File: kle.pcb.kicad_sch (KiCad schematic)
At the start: 191 parts, among them J2 Conn_02x03_Odd_Even, K0 Esc, K1 F1, K10 F10, K11 F11, K12 F12, K13 PrtSc,NmLk, K14 Pause,ScrLk, K15 Delete,Insert, K16 ~~,`, K17 !,1, K18 @,2, K19 #,3, K2 F2, K20 $,4, K21 %,5, K22 ^,6, K23 &,7, K24 *,8, K25 (,9, K26 ),0, K27 _,-, K28 +,=, K29 Backspace, K3 F3, K30 Home, K31 Tab, K32 Q, K33 W, K34 E, K35 R, K36 T, K37 Y, K38 U, K39 I, K4 F4, K40 O, K41 P, K42 {,[, K43 },], K44 |,\, K45 Page Up, K46 Caps Lock, K47 A, K48 S, K49 D, K5 F5, K50 F, K51 G, K52 H, K53 J, K54 K, K55 L, K56 :,;, K57 ",', K58 Enter, K59 Page Down, K6 F6, K60 Shift, K61 Z, K62 X, K63 C, K64 V, K65 B, K66 N, K67 M, K68 <,,, K69 >,., K7 F7, K70 ?,/, K71 Shift, K72 ↑, K73 End, K74 Ctrl, K75 Win, K76 Alt, K77 Blank, K78 Alt, K79 Fn, K8 F8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

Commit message: initial commit
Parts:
- K77: value Blank -> Space
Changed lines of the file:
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@@
 			)
 		)
-		(property "Value" "Blank"
+		(property "Value" "Space"
 			(at 160.02 92.71 0)
 			(effects

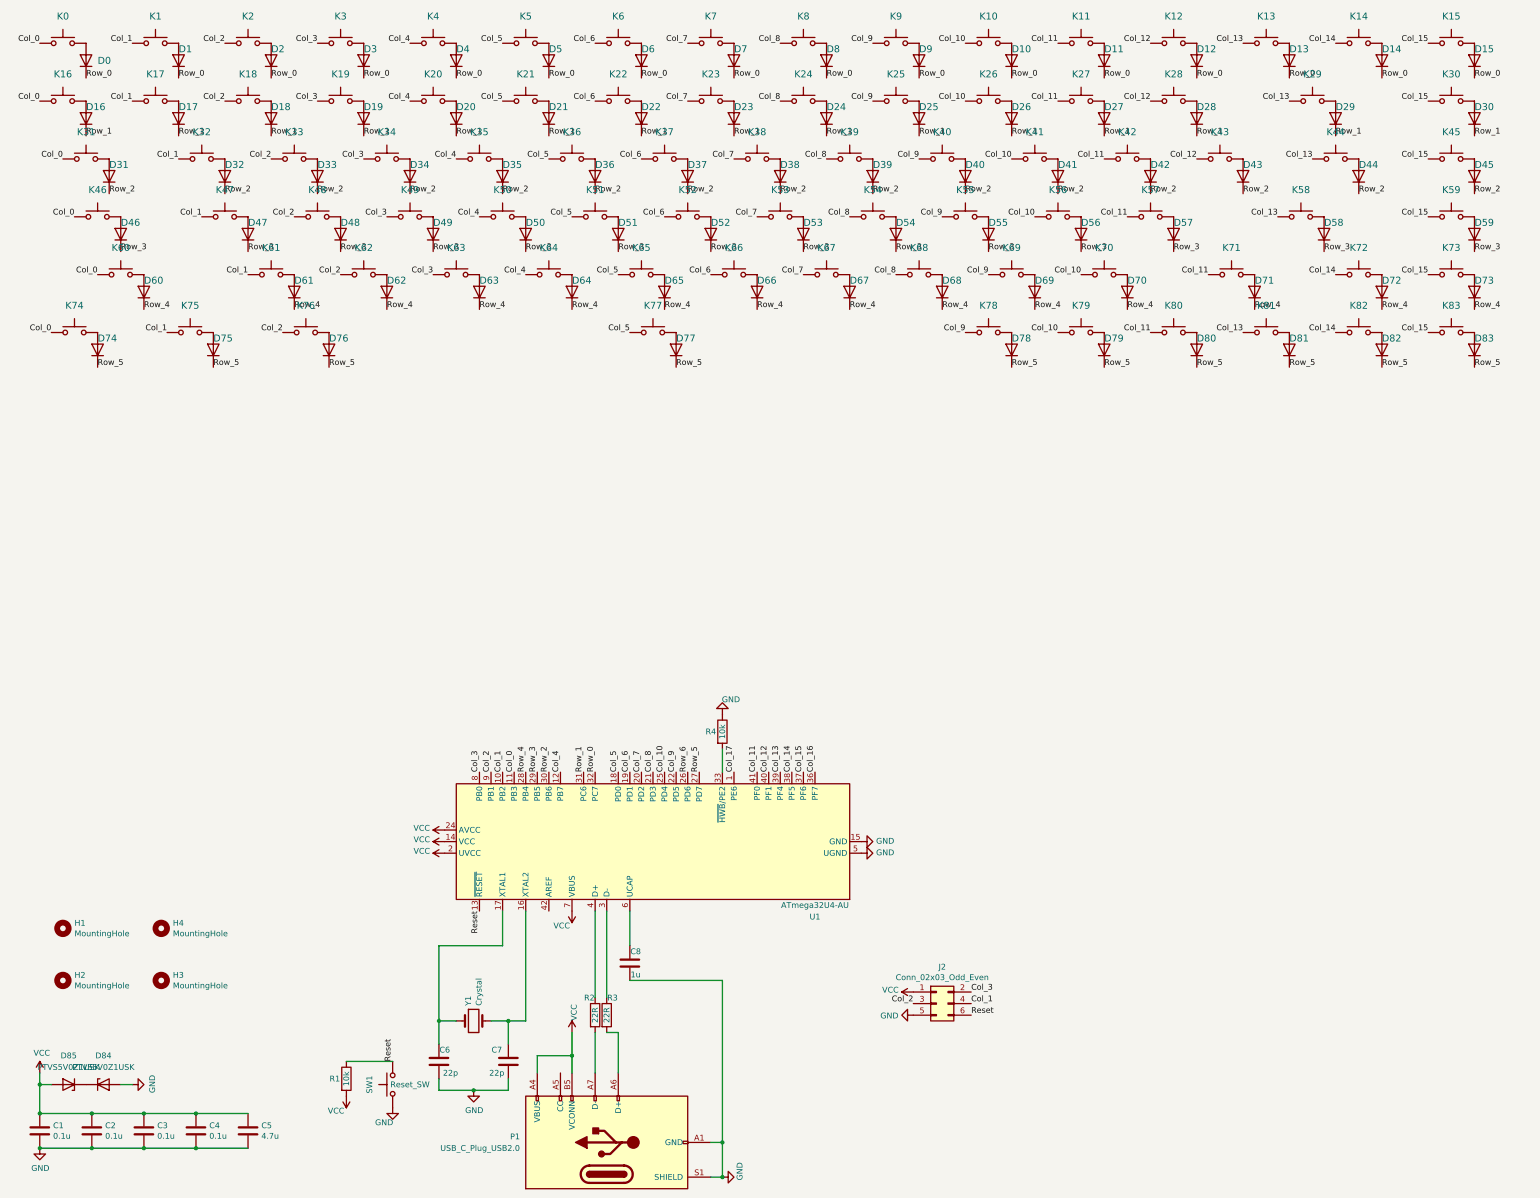
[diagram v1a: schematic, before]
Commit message: progress
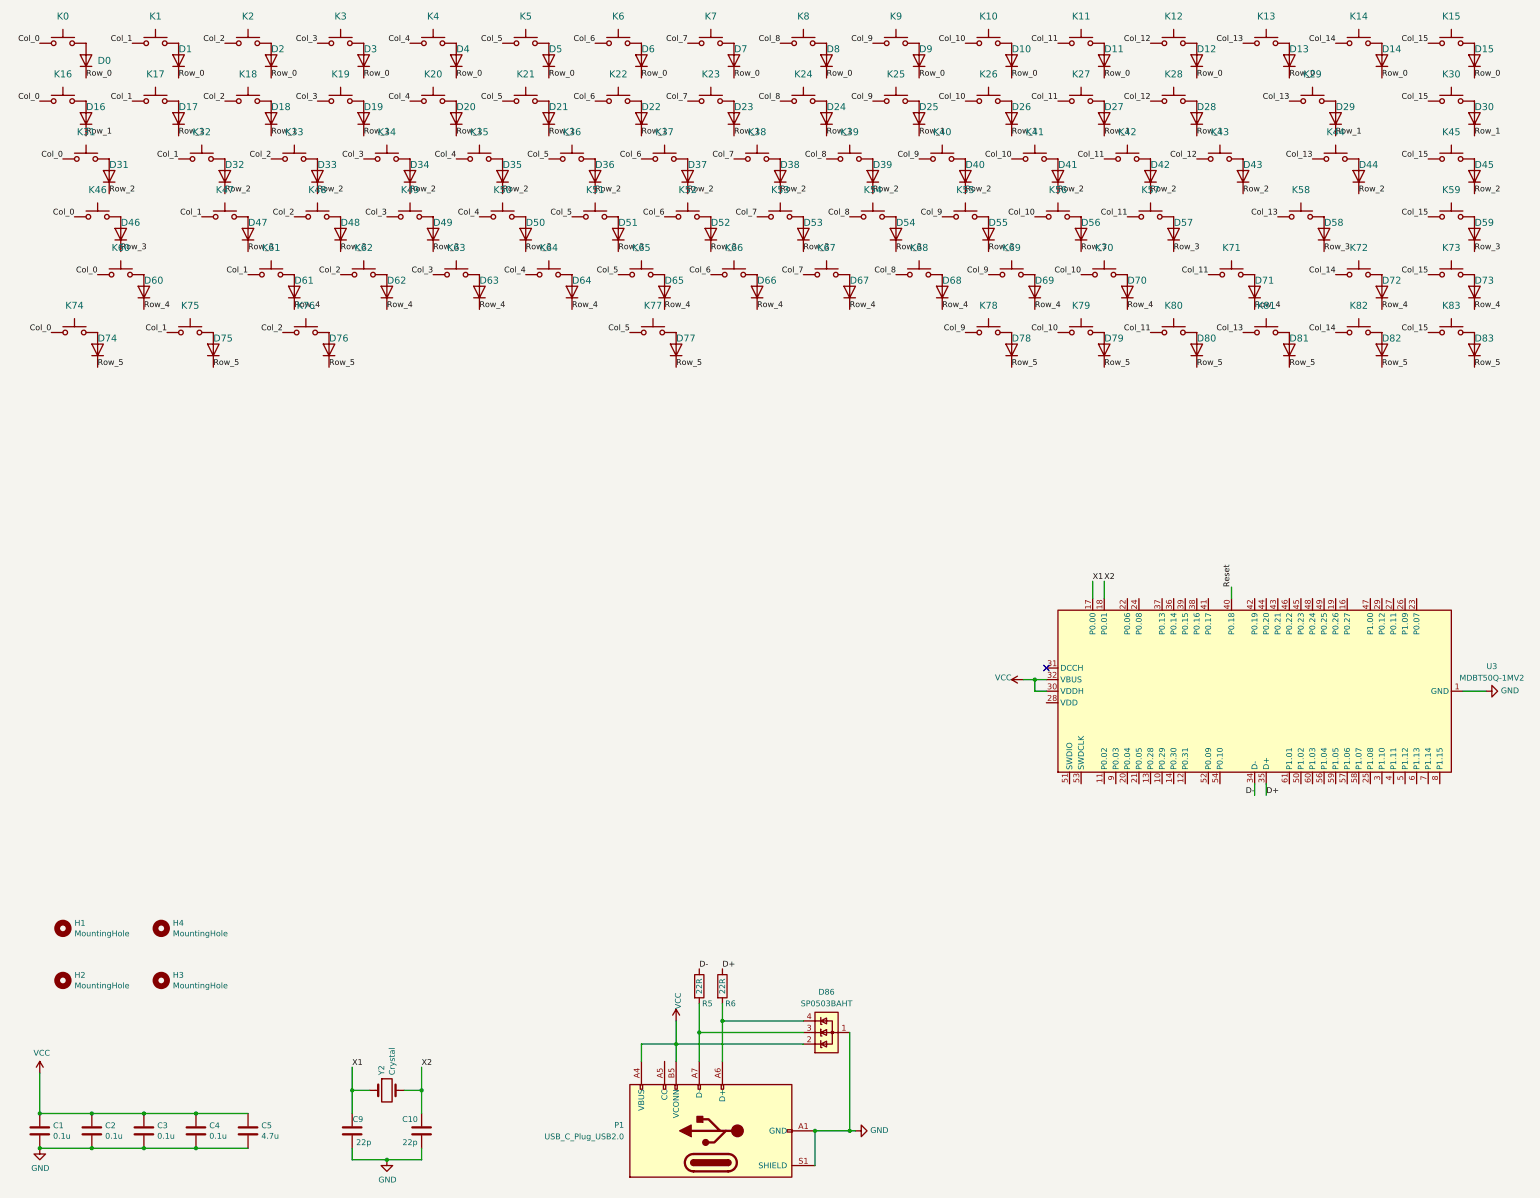
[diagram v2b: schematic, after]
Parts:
- removed C6, C7: 22p, Capacitor_SMD:C_0805_2012Metric_Pad1.15x1.40mm_HandSolder, symbol Device:C
- removed C8: 1u, Capacitor_SMD:C_0805_2012Metric_Pad1.15x1.40mm_HandSolder, symbol Device:C
- removed D84, D85: PTVS5V0Z1USK, Diode_SMD:Nexperia_DSN1608-2_1.6x0.8mm, symbol Diode:PTVS5V0Z1USK
- removed J2: Conn_02x03_Odd_Even, Connector_PinHeader_2.54mm:PinHeader_2x03_P2.54mm_Vertical, symbol Connector_Generic:Conn_02x03_Odd_Even
- removed R1, R4: 10k, Resistor_SMD:R_0805_2012Metric_Pad1.15x1.40mm_HandSolder, symbol Device:R
- removed R2, R3: 22R, Resistor_SMD:R_0805_2012Metric_Pad1.15x1.40mm_HandSolder, symbol Device:R
- removed SW1: Reset_SW, Button_Switch_SMD:SW_Push_1P1T_NO_6x6mm_H9.5mm, symbol Switch:SW_Push
- removed U1: ATmega32U4-AU, Package_QFP:TQFP-44_10x10mm_P0.8mm, symbol MCU_Microchip_ATmega:ATmega32U4-A
- removed Y1: Crystal, Crystal:Crystal_SMD_5032-2Pin_5.0x3.2mm_HandSoldering, symbol Device:Crystal
- added C10, C9: 22p, Capacitor_SMD:C_0805_2012Metric_Pad1.15x1.40mm_HandSolder, symbol Device:C
- added D86: SP0503BAHT, Package_TO_SOT_SMD:SOT-143, symbol Power_Protection:SP0503BAHT
- added R5, R6: 22R, Resistor_SMD:R_0805_2012Metric_Pad1.20x1.40mm_HandSolder, symbol Device:R
- added U3: MDBT50Q-1MV2, RF_Module:Raytac_MDBT50Q, symbol RF_Module:MDBT50Q-1MV2
- added Y2: Crystal, Crystal:Crystal_SMD_5032-2Pin_5.0x3.2mm_HandSoldering, symbol Device:Crystal
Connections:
- net GND: now also C10.2, C9.2, D86.1 (A), U3.1 (GND), U3.15 (GND), U3.2 (GND), U3.33 (GND), U3.55 (GND)
- net Reset: now also U3.40 (P0.18)
- net VCC: now also D86.2 (K), U3.30 (VDDH), U3.32 (VBUS)
- net at P1.A7 (D-): now also D86.3 (K), R5.2
- net at P1.A6 (D+): now also D86.4 (K), R6.2
- new net D+: R6.1, U3.35 (D+)
- new net D-: R5.1, U3.34 (D-)
- new net X1: C9.1, U3.17 (P0.00), Y2.1
- new net X2: C10.1, U3.18 (P0.01), Y2.2
- no-connect marks 0 -> 1
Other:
- moved on the sheet: P1
